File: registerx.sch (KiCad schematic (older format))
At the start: 6 parts, among them U11 74LS245, U12 74LS173, U13 74LS173, U14 74LS245, U15 74LS173, U16 74LS173

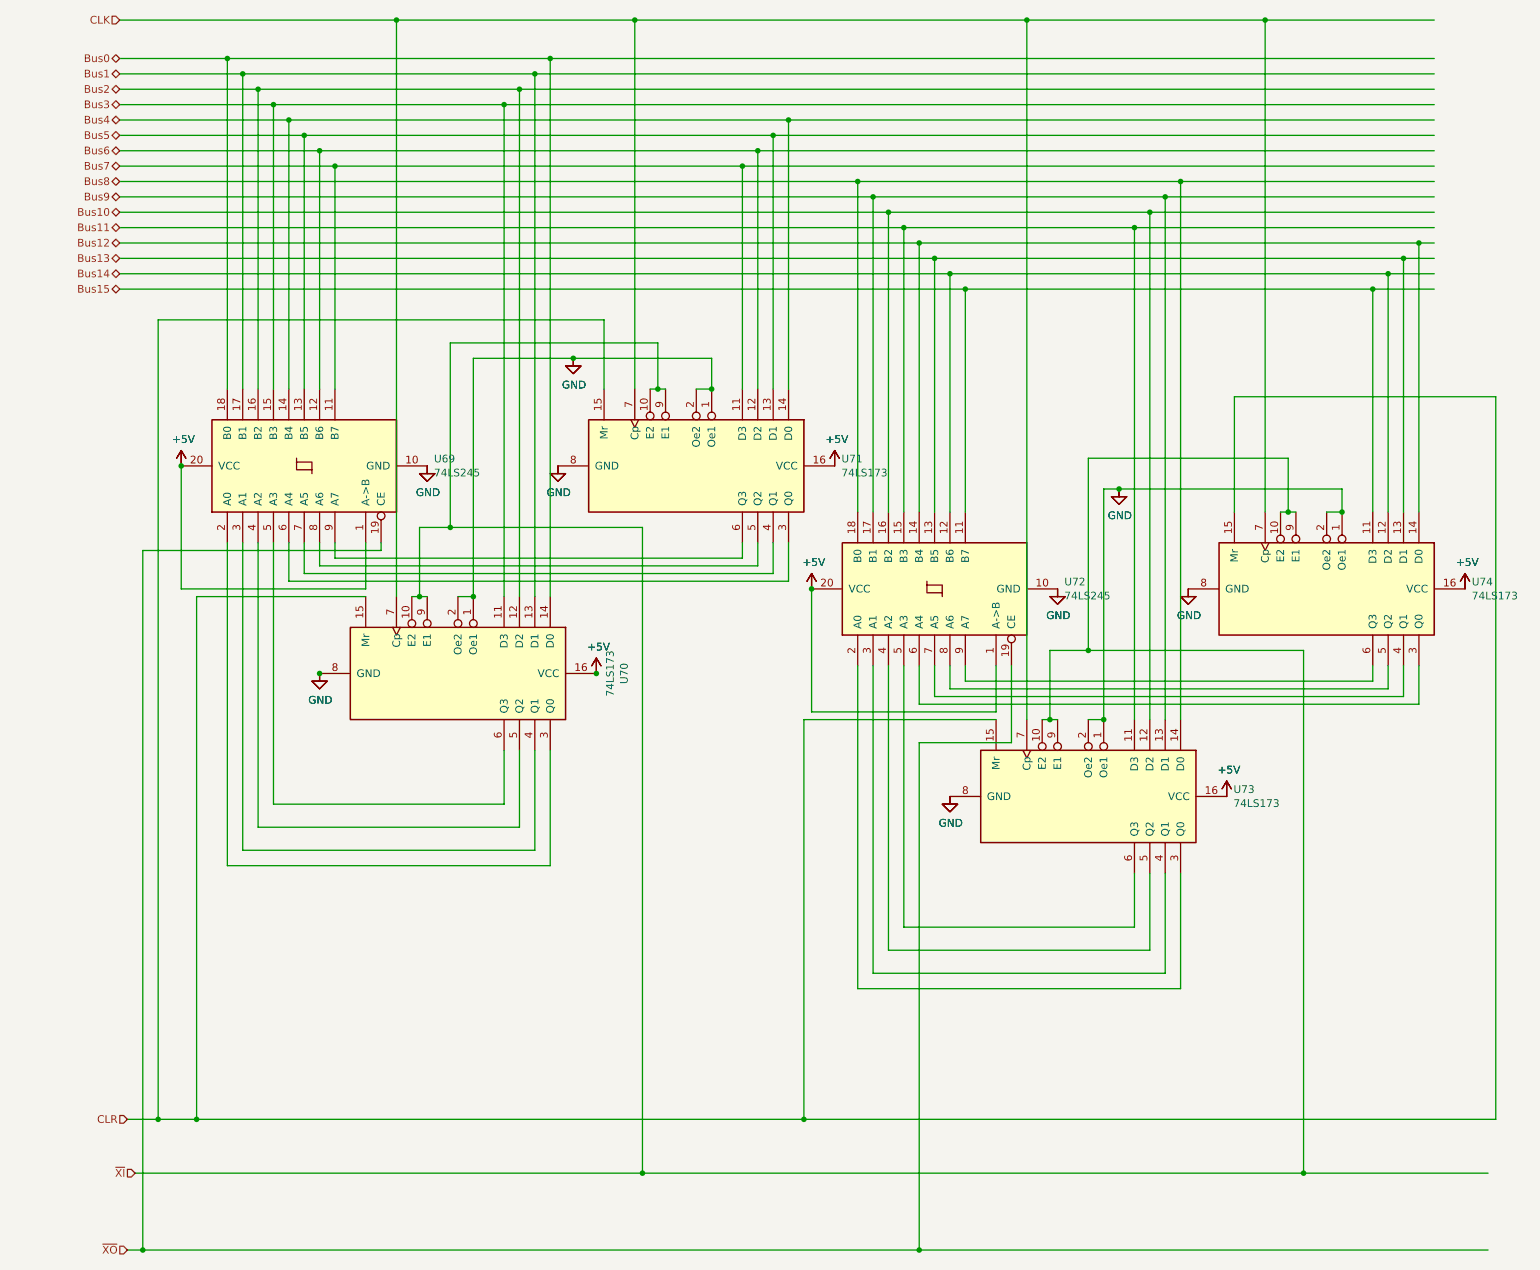
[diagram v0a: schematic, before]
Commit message: Let there be light
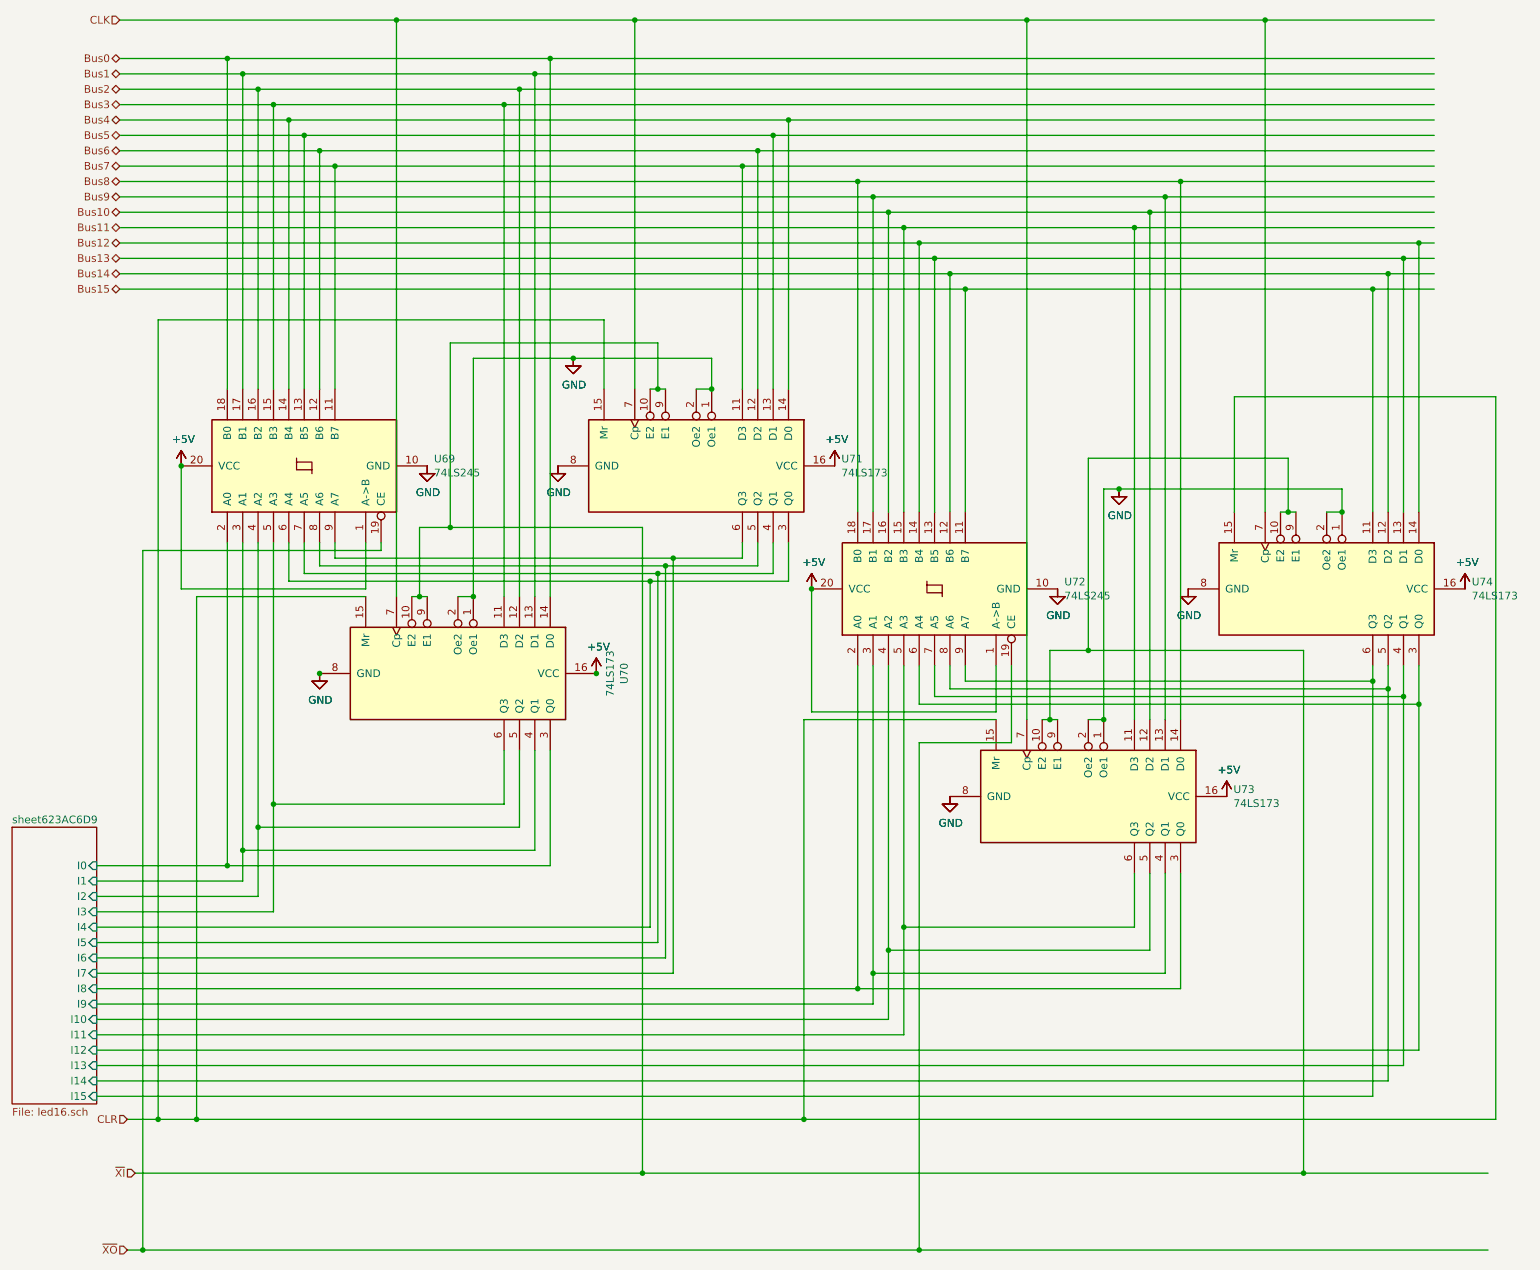
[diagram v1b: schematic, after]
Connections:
- wire segments 203 -> 237
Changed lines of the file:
@@
 $Descr A3 16535 11693
 encoding utf-8
-Sheet 11 11
+Sheet 18 20
 Title ""
 Date ""
@@
 	6400 6500 7900 6500
 Wire Wire Line
-	2700 4100 5350 4100
-Wire Wire Line
-	2600 4150 5450 4150
-Wire Wire Line
-	2400 4250 5650 4250
-Wire Wire Line
-	2500 4200 5550 4200
+	2700 4100 4900 4100
+Wire Wire Line
+	2600 4150 4850 4150
+Wire Wire Line
+	2400 4250 4750 4250
+Wire Wire Line
+	2500 4200 4800 4200
 Wire Wire Line
 	2000 6100 4100 6100
@@
 Wire Wire Line
 	2300 5700 3800 5700
+$Sheet
+S 600  5850 550  1800
+U 623AC6EB
+F0 "sheet623AC6D9" 50
+F1 "led16.sch" 50
+F2 "I0" I R 1150 6100 50
+F3 "I1" I R 1150 6200 50
+F4 "I2" I R 1150 6300 50
+F5 "I3" I R 1150 6400 50
+F6 "I4" I R 1150 6500 50
+F7 "I5" I R 1150 6600 50
+F8 "I6" I R 1150 6700 50
+F9 "I7" I R 1150 6800 50
+F10 "I8" I R 1150 6900 50
+F11 "I9" I R 1150 7000 50
+F12 "I10" I R 1150 7100 50
+F13 "I11" I R 1150 7200 50
+F14 "I12" I R 1150 7300 50
+F15 "I13" I R 1150 7400 50
+F16 "I14" I R 1150 7500 50
+F17 "I15" I R 1150 7600 50
+$EndSheet
+Wire Wire Line
+	1150 6100 2000 6100
+Connection ~ 2000 6100
+Wire Wire Line
+	2100 6000 2100 6200
+Wire Wire Line
+	2100 6200 1150 6200
+Connection ~ 2100 6000
+Wire Wire Line
+	1150 6300 2200 6300
+Wire Wire Line
+	2200 6300 2200 5850
+Connection ~ 2200 5850
+Wire Wire Line
+	2300 5700 2300 6400
+Wire Wire Line
+	2300 6400 1150 6400
+Connection ~ 2300 5700
+Wire Wire Line
+	1150 6500 4750 6500
+Wire Wire Line
+	4750 6500 4750 4250
+Connection ~ 4750 4250
+Wire Wire Line
+	4750 4250 5650 4250
+Wire Wire Line
+	1150 6600 4800 6600
+Wire Wire Line
+	4800 6600 4800 4200
+Connection ~ 4800 4200
+Wire Wire Line
+	4800 4200 5550 4200
+Wire Wire Line
+	1150 6700 4850 6700
+Wire Wire Line
+	4850 6700 4850 4150
+Connection ~ 4850 4150
+Wire Wire Line
+	4850 4150 5450 4150
+Wire Wire Line
+	1150 6800 4900 6800
+Wire Wire Line
+	4900 6800 4900 4100
+Connection ~ 4900 4100
+Wire Wire Line
+	4900 4100 5350 4100
+Wire Wire Line
+	1150 6900 6100 6900
+Connection ~ 6100 6900
+Wire Wire Line
+	6200 6800 6200 7000
+Wire Wire Line
+	6200 7000 1150 7000
+Connection ~ 6200 6800
+Wire Wire Line
+	1150 7100 6300 7100
+Wire Wire Line
+	6300 7100 6300 6650
+Connection ~ 6300 6650
+Wire Wire Line
+	1150 7200 6400 7200
+Wire Wire Line
+	6400 7200 6400 6500
+Connection ~ 6400 6500
+Wire Wire Line
+	1150 7300 9750 7300
+Wire Wire Line
+	9750 7300 9750 5050
+Connection ~ 9750 5050
+Wire Wire Line
+	9650 5000 9650 7400
+Wire Wire Line
+	9650 7400 1150 7400
+Connection ~ 9650 5000
+Wire Wire Line
+	1150 7500 9550 7500
+Wire Wire Line
+	9550 7500 9550 4950
+Connection ~ 9550 4950
+Wire Wire Line
+	9450 4900 9450 7600
+Wire Wire Line
+	9450 7600 1150 7600
+Connection ~ 9450 4900
 $EndSCHEMATC
